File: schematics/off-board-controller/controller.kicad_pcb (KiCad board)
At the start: 2 copper layers, 110 x 90 mm, 70 parts, among them J1 programmer, J2 5-1814832-1, J3 9V, SW5 SW_SPDT_MSM, U4 STM32L476RGTx, U5 RFM98W-433S2, U6 L78L33_TO92, U8 MCP23S17_SP, U9 MCP23S17_SP

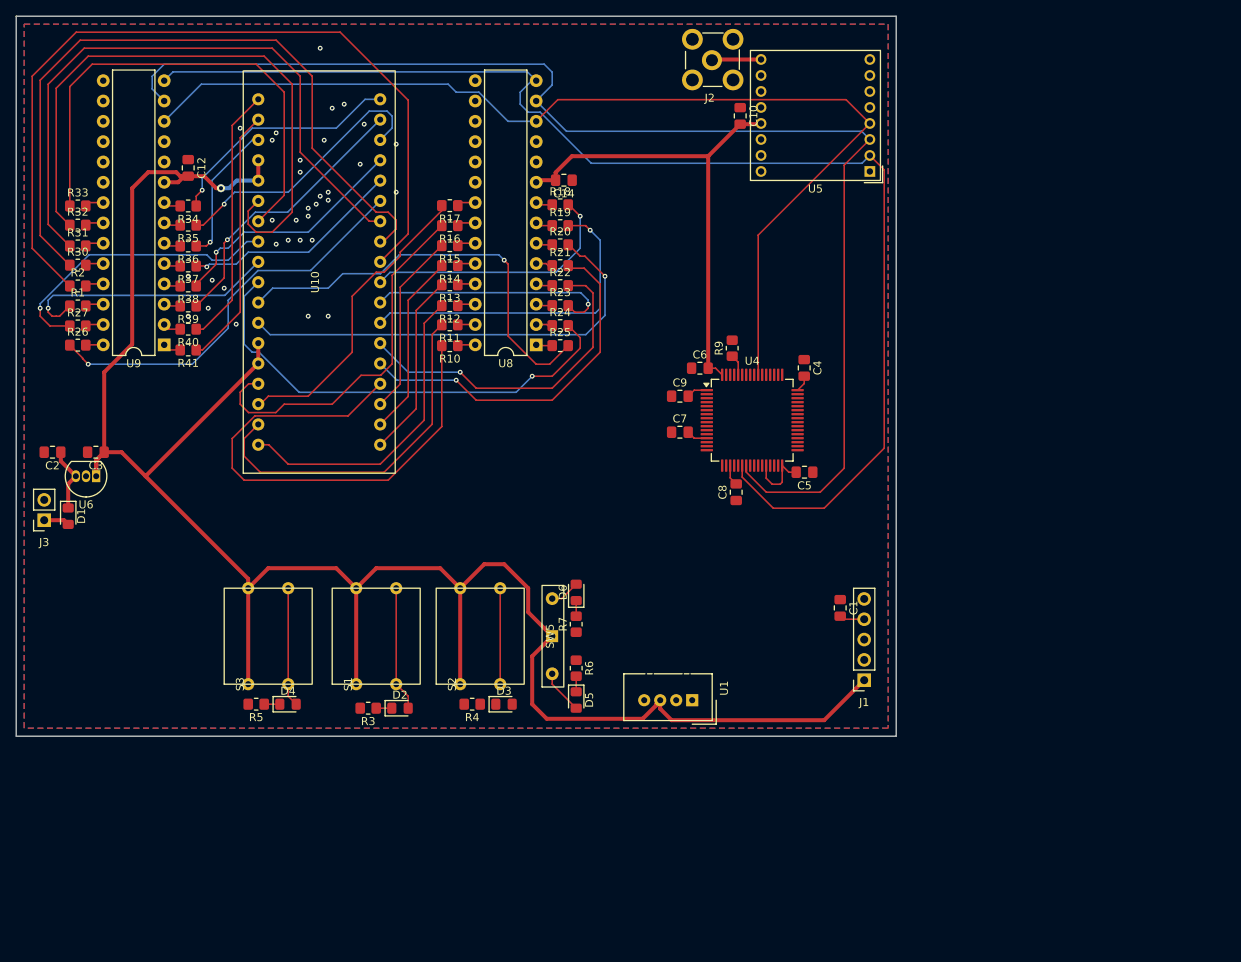
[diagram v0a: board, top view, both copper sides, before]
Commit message: redesigned layout
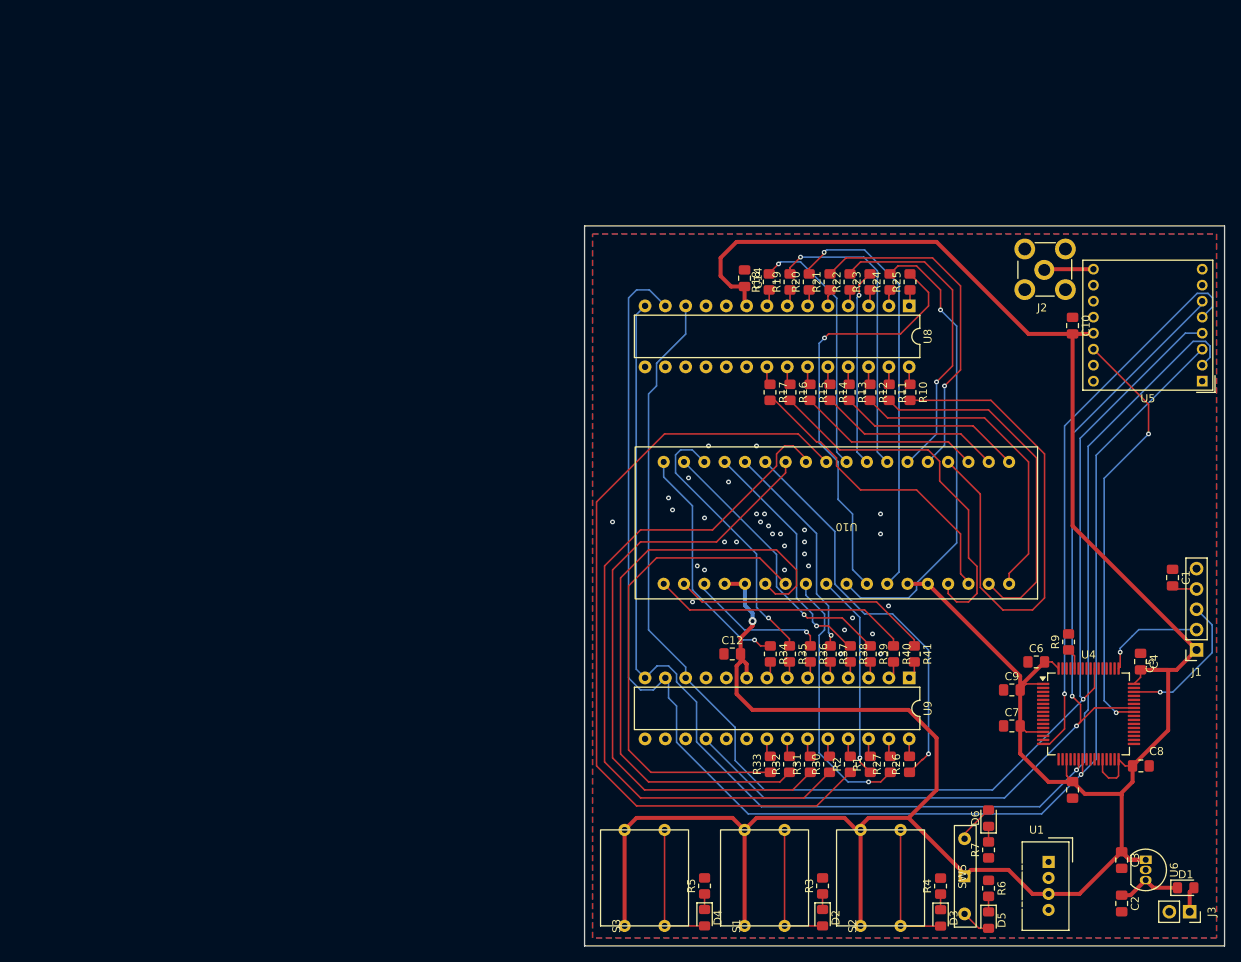
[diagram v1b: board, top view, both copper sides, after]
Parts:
- moved J3 151.3 mm to (165.7, 132.9), turned to -90 degrees
- moved D1 147.2 mm to (165.2, 129.9), turned to 0 degrees
- moved C2 145.1 mm to (157.2, 131.9), turned to -90 degrees
- moved U6 139.7 mm to (160.2, 126.4), turned to -90 degrees
- moved C3 138.0 mm to (157.2, 126.5), turned to -90 degrees
- moved R26 116.4 mm to (130.7, 114.5), turned to 90 degrees
- moved R27 115.4 mm to (128.3, 114.5), turned to 90 degrees
- moved R1 114.4 mm to (125.8, 114.5), turned to 90 degrees
- moved R2 113.6 mm to (123.3, 114.5), turned to 90 degrees
- moved R30 112.8 mm to (120.7, 114.5), turned to 90 degrees
- moved R31 112.2 mm to (118.3, 114.5), turned to 90 degrees
- moved R32 111.6 mm to (115.7, 114.5), turned to 90 degrees
- moved R33 111.2 mm to (113.3, 114.5), turned to 90 degrees
- moved U9 102.0 mm to (130.6, 103.7), turned to -90 degrees
- moved R41 98.4 mm to (131.3, 100.7), turned to -90 degrees
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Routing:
- net RESET_IO: track 0.00 -> 121.7 mm, vias 0 -> 2
- net CS_RADIO: track 0.00 -> 69.9 mm, vias 0 -> 1
- net +3V3: track 332.5 -> 387.2 mm
- net RADIO_DONE: track 0.00 -> 53.5 mm, vias 0 -> 2
- net SCK: track 131.6 -> 170.9 mm, vias 0 -> 1
- net MOSI: track 160.6 -> 185.5 mm, vias 0 -> 1
- net MISO: track 159.9 -> 180.9 mm, vias 0 -> 1
- net /mcu/SWDIO: track 0.00 -> 18.1 mm, vias 0 -> 1
- net /mcu/SWCLK: track 0.00 -> 13.1 mm, vias 0 -> 1
- net Net-(U10-3f): track 33.2 -> 25.8 mm
- net Net-(U10-2c): track 30.9 -> 24.7 mm
- net BTN_REQ_CODE: track 12.0 -> 17.0 mm
- net Net-(U10-2g): track 41.5 -> 37.4 mm
- net Net-(U10-3g): track 36.8 -> 33.3 mm
- net Net-(U10-2f): track 56.1 -> 52.8 mm
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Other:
- board size 110 x 90 mm -> 80 x 90 mm
